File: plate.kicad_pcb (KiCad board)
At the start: 2 copper layers, 149.8 x 115.9 mm, 35 parts, among them SW1 ESC, SW10 E, SW11 R, SW12 T, SW13 CAPS, SW14 A, SW15 S, SW16 D, SW17 F, SW18 G, SW19 SHIFT, SW2 1, SW20 <, SW21 Z, SW22 X, SW23 C, SW24 V, SW25 CTRL, SW26 SUPER, SW27 ALT, SW28 X, SW29 C, SW3 2, SW30 Rotary_Encoder_Switch, SW4 3, SW5 4, SW6 5, SW7 TAB, SW8 Q, SW9 W

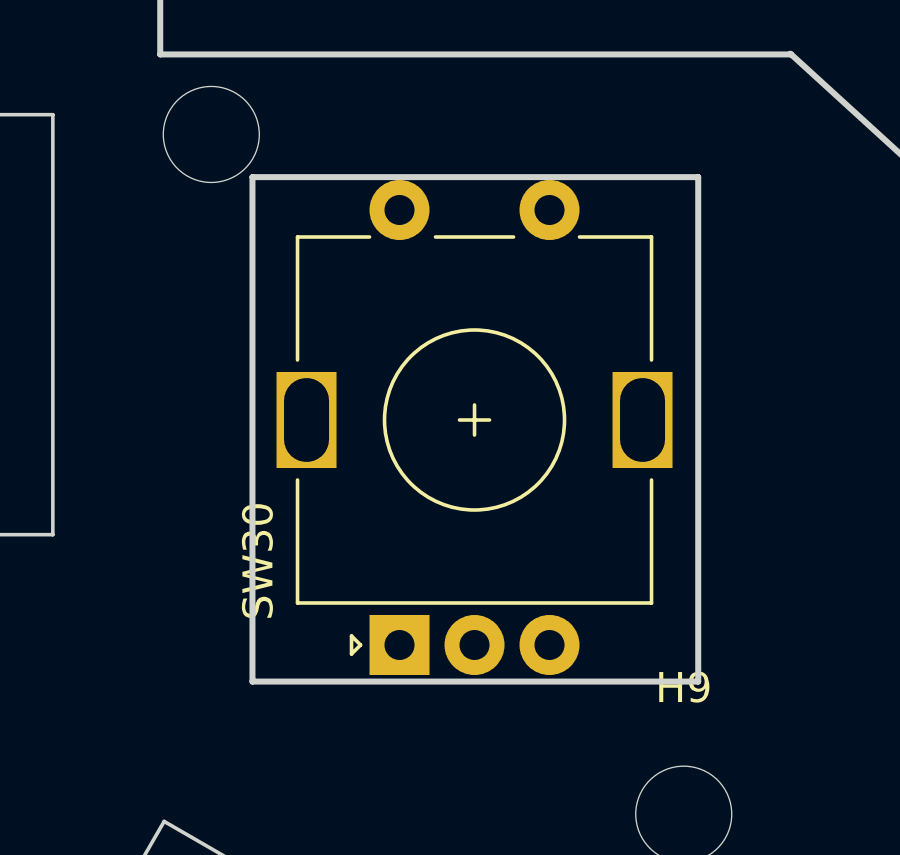
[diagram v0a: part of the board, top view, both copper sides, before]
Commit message: More gerbers
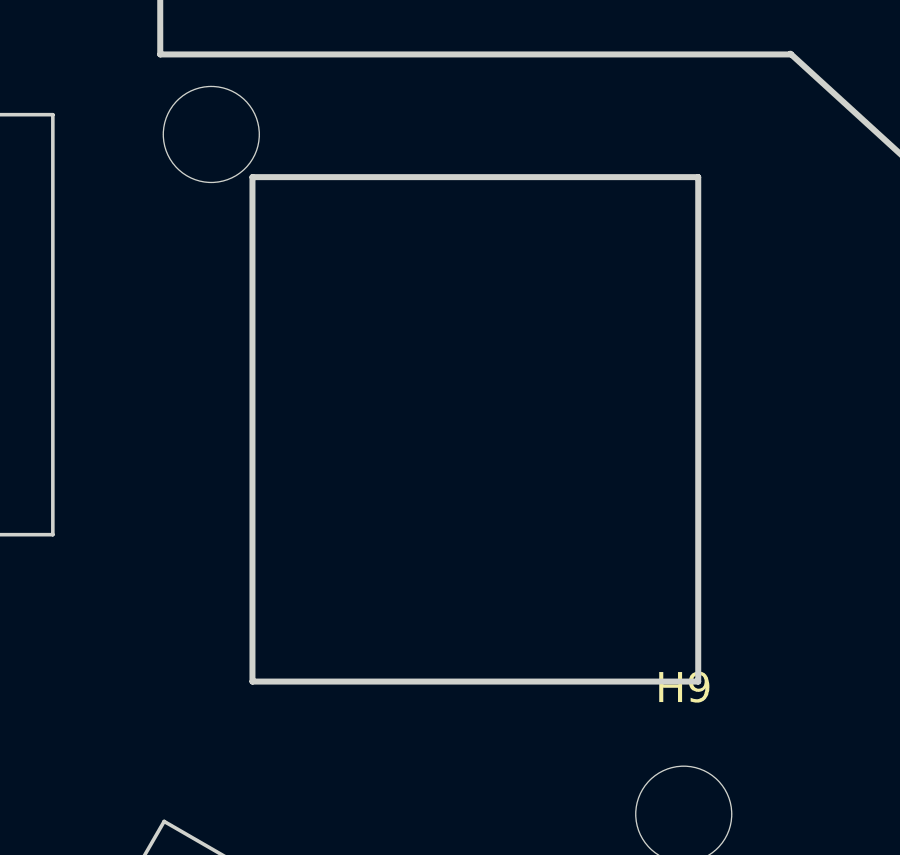
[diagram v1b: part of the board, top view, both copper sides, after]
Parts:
- removed SW30: Rotary_Encoder_Switch, Rotary_Encoder:RotaryEncoder_Alps_EC11E-Switch_Vertical_H20mm
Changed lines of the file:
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@@
     (tracks 2)
     (zones 0)
-    (modules 35)
-    (nets 7)
+    (modules 34)
+    (nets 3)
   )
   (page A4)
   (layers
-    (0 F.Cu signal hide)
+    (0 F.Cu signal)
     (31 B.Cu signal hide)
     (32 B.Adhes user hide)
@@
     (visible_elements FFFFFF7F)
     (pcbplotparams
-      (layerselection 0x01000_7ffffffe)
+      (layerselection 0x010f0_ffffffff)
       (usegerberextensions false)
       (usegerberattributes false)
@@
       (padsonsilk false)
       (subtractmaskfromsilk false)
-      (outputformat 4)
+      (outputformat 1)
       (mirror false)
       (drillshape 0)
       (scaleselection 1)
-      (outputdirectory "/home/thys/Public/"))
+      (outputdirectory "gerbers-plate/"))
   )
   (net 0 "")
   (net 1 GND)
   (net 2 col3)
-  (net 3 col5)
-  (net 4 ROT1A)
-  (net 5 ROT1B)
-  (net 6 "Net-(D30-Pad2)")
   (net_class Default "This is the default net class."
     (clearance 0.2)
@@
     (uvia_dia 0.3)
     (uvia_drill 0.1)
-    (add_net GND)
-    (add_net "Net-(D30-Pad2)")
-    (add_net ROT1A)
-    (add_net ROT1B)
     (add_net col3)
-    (add_net col5)
   )
   (module MountingHole:MountingHole_3.2mm_M3 (layer F.Cu)
@@
     (pad 1 np_thru_hole circle (at 0 0) (size 3.2 3.2) (drill 3.2) (layers *.Cu *.Mask))
   )
-  (module Rotary_Encoder:RotaryEncoder_Alps_EC11E-Switch_Vertical_H20mm (layer F.Cu)
-    (at 178.765 126.67 90)
-    (descr "Alps rotary encoder, EC12E... with switch, vertical shaft, http://www.alps.com/prod/info/E/HTML/Encoder/Incremental/EC11/EC11E15204A3.html")
-    (tags "rotary encoder")
-    (fp_text reference SW30 (at 2.8 -4.7 90) (layer F.SilkS)
-      (effects (font (size 1 1) (thickness 0.15)))
-    )
-    (fp_text value Rotary_Encoder_Switch (at 7.5 10.4 90) (layer F.Fab)
-      (effects (font (size 1 1) (thickness 0.15)))
-    )
-    (fp_circle (center 7.5 2.5) (end 10.5 2.5) (layer F.Fab) (width 0.12))
-    (fp_circle (center 7.5 2.5) (end 10.5 2.5) (layer F.SilkS) (width 0.12))
-    (fp_line (start 16 9.6) (end -1.5 9.6) (layer F.CrtYd) (width 0.05))
-    (fp_line (start 16 9.6) (end 16 -4.6) (layer F.CrtYd) (width 0.05))
-    (fp_line (start -1.5 -4.6) (end -1.5 9.6) (layer F.CrtYd) (width 0.05))
-    (fp_line (start -1.5 -4.6) (end 16 -4.6) (layer F.CrtYd) (width 0.05))
-    (fp_line (start 2.5 -3.3) (end 13.5 -3.3) (layer F.Fab) (width 0.12))
-    (fp_line (start 13.5 -3.3) (end 13.5 8.3) (layer F.Fab) (width 0.12))
-    (fp_line (start 13.5 8.3) (end 1.5 8.3) (layer F.Fab) (width 0.12))
-    (fp_line (start 1.5 8.3) (end 1.5 -2.2) (layer F.Fab) (width 0.12))
-    (fp_line (start 1.5 -2.2) (end 2.5 -3.3) (layer F.Fab) (width 0.12))
-    (fp_line (start 9.5 -3.4) (end 13.6 -3.4) (layer F.SilkS) (width 0.12))
-    (fp_line (start 13.6 8.4) (end 9.5 8.4) (layer F.SilkS) (width 0.12))
-    (fp_line (start 5.5 8.4) (end 1.4 8.4) (layer F.SilkS) (width 0.12))
-    (fp_line (start 5.5 -3.4) (end 1.4 -3.4) (layer F.SilkS) (width 0.12))
-    (fp_line (start 1.4 -3.4) (end 1.4 8.4) (layer F.SilkS) (width 0.12))
-    (fp_line (start 0 -1.3) (end -0.3 -1.6) (layer F.SilkS) (width 0.12))
-    (fp_line (start -0.3 -1.6) (end 0.3 -1.6) (layer F.SilkS) (width 0.12))
-    (fp_line (start 0.3 -1.6) (end 0 -1.3) (layer F.SilkS) (width 0.12))
-    (fp_line (start 7.5 -0.5) (end 7.5 5.5) (layer F.Fab) (width 0.12))
-    (fp_line (start 4.5 2.5) (end 10.5 2.5) (layer F.Fab) (width 0.12))
-    (fp_line (start 13.6 -3.4) (end 13.6 -1) (layer F.SilkS) (width 0.12))
-    (fp_line (start 13.6 1.2) (end 13.6 3.8) (layer F.SilkS) (width 0.12))
-    (fp_line (start 13.6 6) (end 13.6 8.4) (layer F.SilkS) (width 0.12))
-    (fp_line (start 7.5 2) (end 7.5 3) (layer F.SilkS) (width 0.12))
-    (fp_line (start 7 2.5) (end 8 2.5) (layer F.SilkS) (width 0.12))
-    (fp_text user %R (at 11.1 6.3 90) (layer F.Fab)
-      (effects (font (size 1 1) (thickness 0.15)))
-    )
-    (pad A thru_hole rect (at 0 0 90) (size 2 2) (drill 1) (layers *.Cu *.Mask)
-      (net 4 ROT1A))
-    (pad C thru_hole circle (at 0 2.5 90) (size 2 2) (drill 1) (layers *.Cu *.Mask)
-      (net 1 GND))
-    (pad B thru_hole circle (at 0 5 90) (size 2 2) (drill 1) (layers *.Cu *.Mask)
-      (net 5 ROT1B))
-    (pad MP thru_hole rect (at 7.5 -3.1 90) (size 3.2 2) (drill oval 2.8 1.5) (layers *.Cu *.Mask))
-    (pad MP thru_hole rect (at 7.5 8.1 90) (size 3.2 2) (drill oval 2.8 1.5) (layers *.Cu *.Mask))
-    (pad S2 thru_hole circle (at 14.5 0 90) (size 2 2) (drill 1) (layers *.Cu *.Mask)
-      (net 3 col5))
-    (pad S1 thru_hole circle (at 14.5 5 90) (size 2 2) (drill 1) (layers *.Cu *.Mask)
-      (net 6 "Net-(D30-Pad2)"))
-    (model ${KISYS3DMOD}/Rotary_Encoder.3dshapes/RotaryEncoder_Alps_EC11E-Switch_Vertical_H20mm.wrl
-      (at (xyz 0 0 0))
-      (scale (xyz 1 1 1))
-      (rotate (xyz 0 0 0))
-    )
-  )
   (module foostan:SW_Hole (layer F.Cu)
